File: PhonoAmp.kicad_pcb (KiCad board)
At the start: 2 copper layers, 143.5 x 76.2 mm, 33 parts, among them J1 Screw_Terminal_01x03, J2 Screw_Terminal_01x03, J3 Screw_Terminal_01x02, U1 NE5532, U2 TL072

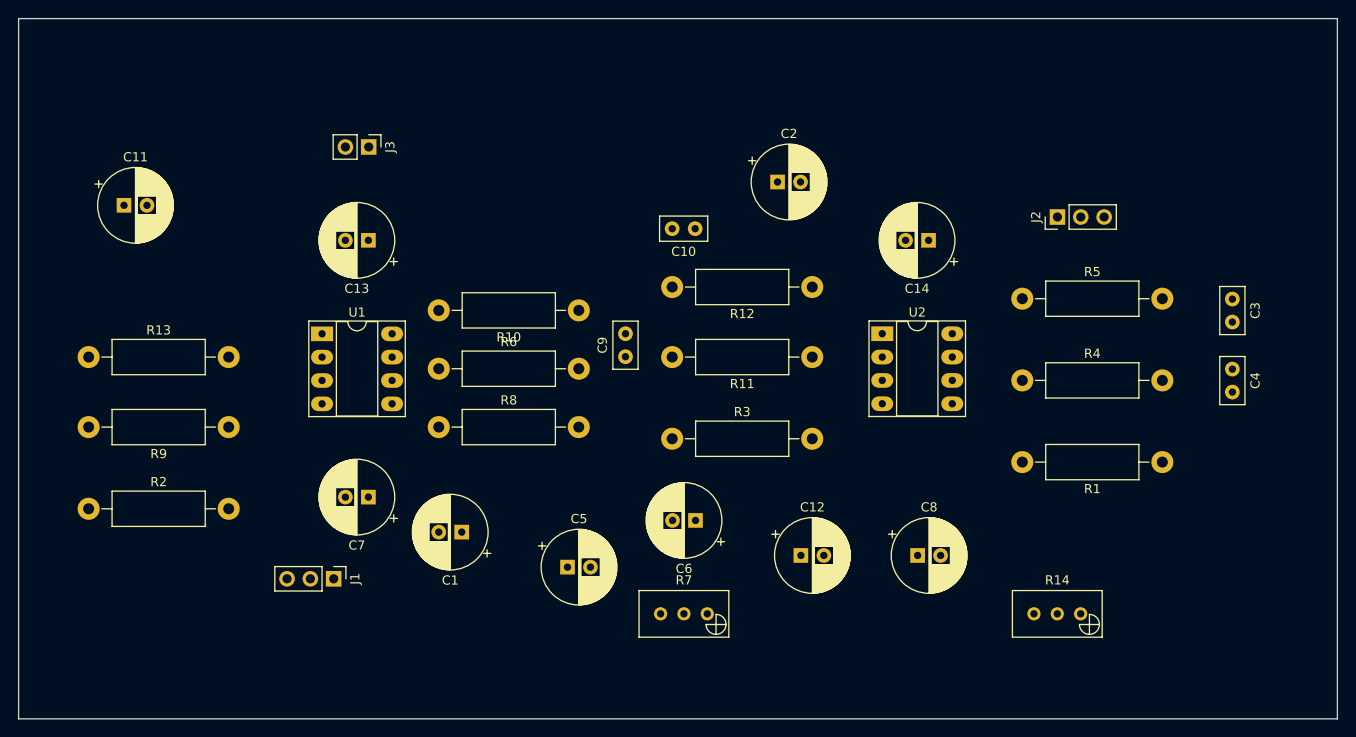
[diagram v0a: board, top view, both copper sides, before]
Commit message: Component Layout reviewed
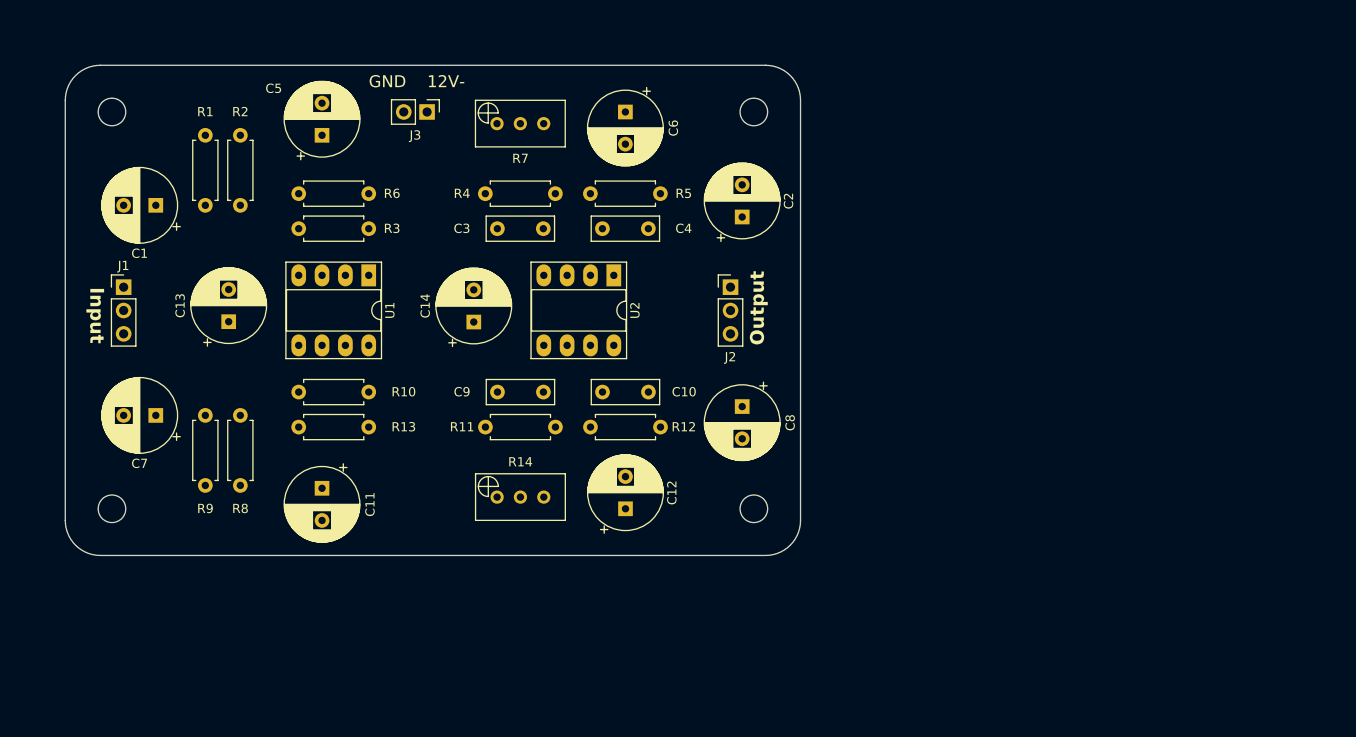
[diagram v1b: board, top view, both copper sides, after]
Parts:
- added H1: MountingHole, MountingHole:MountingHole_3mm, F.Cu at (91.4, 69.8)
- added H2: MountingHole, MountingHole:MountingHole_3mm, F.Cu at (161.3, 69.8)
- added H3: MountingHole, MountingHole:MountingHole_3mm, F.Cu at (91.4, 113.0)
- added H4: MountingHole, MountingHole:MountingHole_3mm, F.Cu at (161.3, 113.0)
- C1, C11, C12, C13, C14, C2, C5, C6, C7, C8: footprint Capacitor_THT:CP_Radial_D8.0mm_P2.50mm -> Capacitor_THT:CP_Radial_D8.0mm_P3.50mm
- C10, C3, C4, C9: footprint Capacitor_THT:C_Disc_D5.0mm_W2.5mm_P2.50mm -> Capacitor_THT:C_Rect_L7.2mm_W2.5mm_P5.00mm_FKS2_FKP2_MKS2_MKP2
- R1, R10, R11, R12, R13, R2, R3, R4, R5, R6, R8, R9: footprint Resistor_THT:R_Axial_DIN0411_L9.9mm_D3.6mm_P15.24mm_Horizontal -> Resistor_THT:R_Axial_DIN0207_L6.3mm_D2.5mm_P7.62mm_Horizontal
- moved R1 107.8 mm to (101.6, 80.0), turned to 90 degrees
- moved C3 75.4 mm to (138.4, 82.5), turned to 180 degrees
- moved C4 65.4 mm to (149.8, 82.5), turned to 180 degrees
- moved R14 64.8 mm to (133.3, 111.8), turned to 180 degrees
- moved R4 61.9 mm to (132.1, 78.7)
- moved R7 58.0 mm to (133.3, 71.1), turned to 180 degrees
- moved C5 54.1 mm to (114.3, 72.4), turned to 90 degrees
- moved C14 50.3 mm to (130.8, 92.7), turned to 90 degrees
- moved C1 48.7 mm to (96.2, 80.0)
- moved C6 45.1 mm to (147.3, 69.8), turned to -90 degrees
- moved R2 43.9 mm to (105.4, 72.4), turned to -90 degrees
- moved R5 41.0 mm to (151.1, 78.7), turned to 180 degrees
- moved R3 40.2 mm to (119.4, 82.5), turned to 180 degrees
- moved J1 39.1 mm to (92.7, 88.9), turned to 0 degrees
- moved C11 37.6 mm to (114.3, 110.8), turned to -90 degrees
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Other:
- board size 143.5 x 76.2 mm -> 80 x 53.3 mm
- board text added: "12V-"
- board text added: "GND"
- board text added: "Input"
- board text added: "Output"

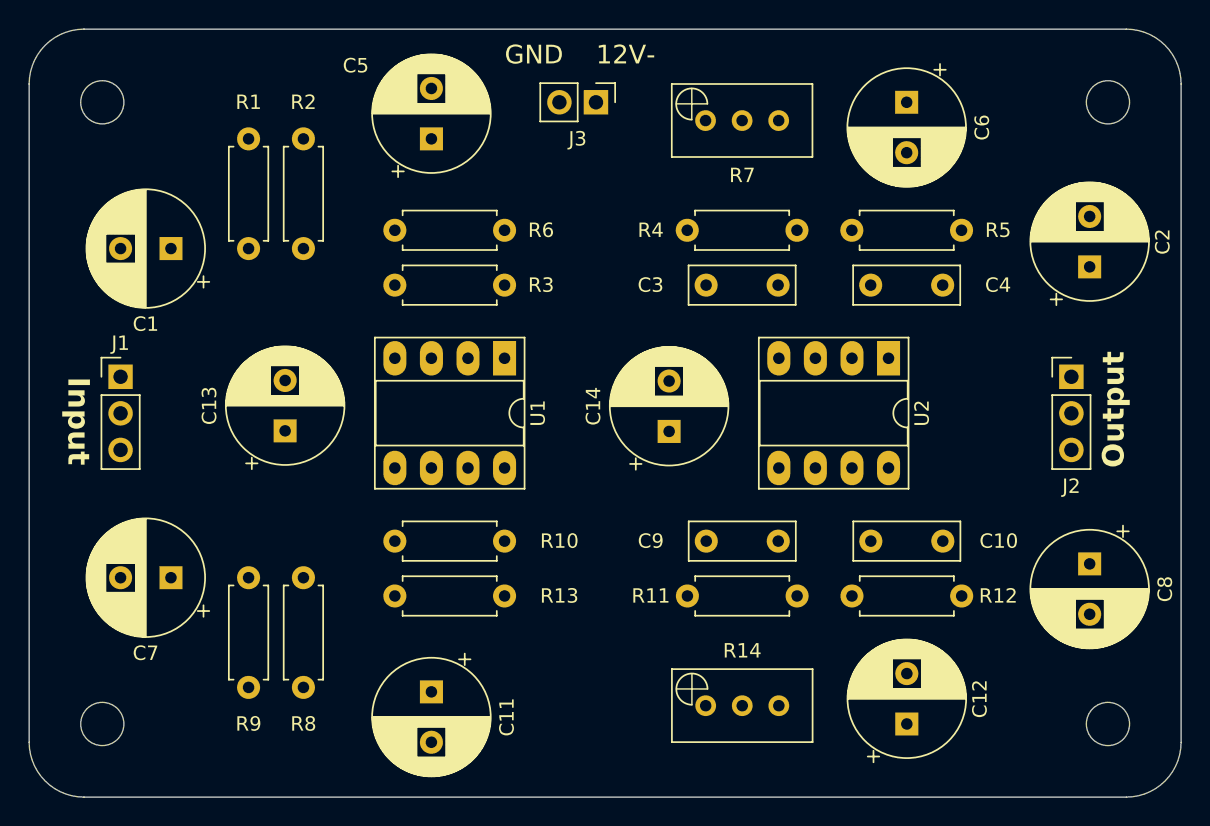
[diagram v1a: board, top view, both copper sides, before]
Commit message: iBom Production files Transferfunctions
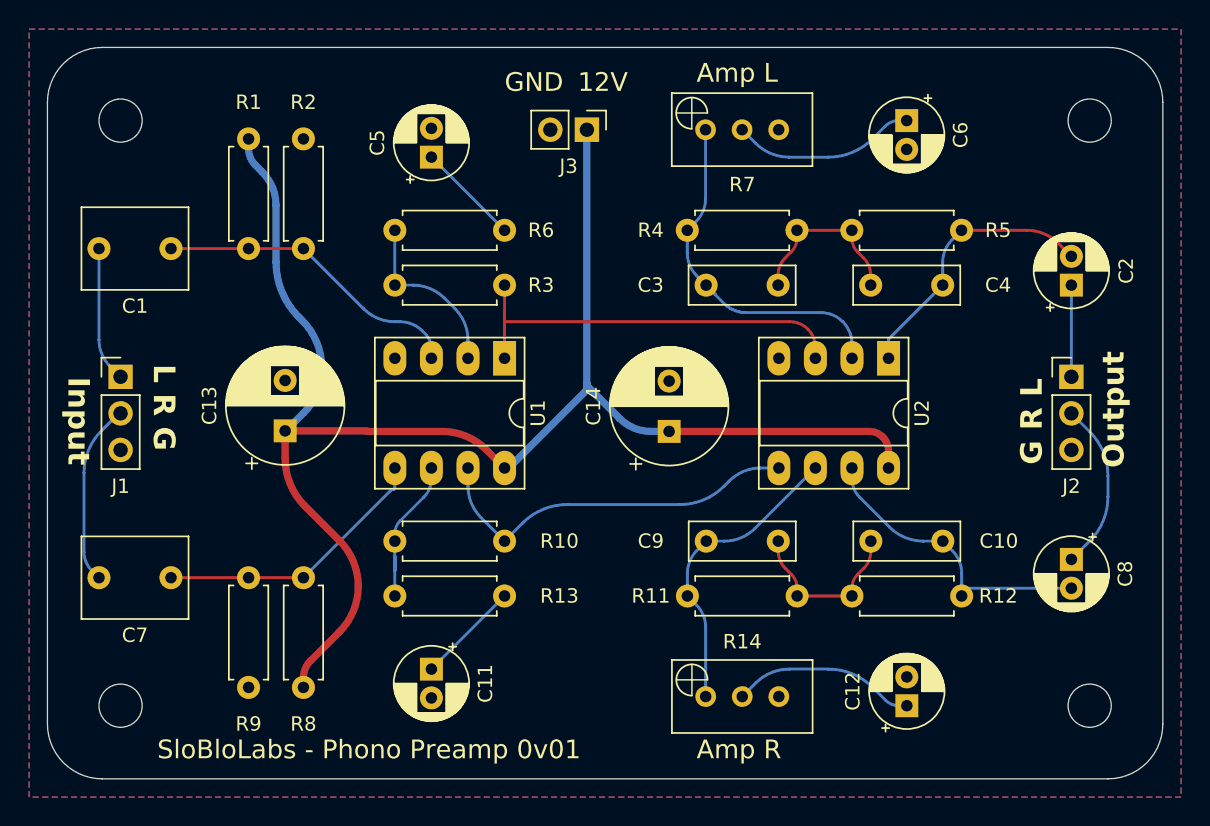
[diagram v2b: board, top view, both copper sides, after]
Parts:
- C1, C7: footprint Capacitor_THT:CP_Radial_D8.0mm_P3.50mm -> Capacitor_THT:C_Rect_L7.2mm_W5.5mm_P5.00mm_FKS2_FKP2_MKS2_MKP2
- C10, C4: value 1n5 -> 1n
- C11, C12, C2, C5, C6, C8: footprint Capacitor_THT:CP_Radial_D8.0mm_P3.50mm -> Capacitor_THT:CP_Radial_D5.0mm_P2.00mm
- C3, C9: value 6n8 -> 10n
- R11, R4: value 750k -> 1M
- moved R3 7.62 mm to (111.8, 82.5), turned to 0 degrees
- moved R6 7.62 mm to (119.4, 78.7), turned to 180 degrees
- moved J3 2.01 mm to (125.1, 71.8)
- moved C2 1.80 mm to (158.8, 82.5)
- moved H1 1.80 mm to (92.7, 71.1)
- moved H3 1.80 mm to (92.7, 111.8)
- moved H2 1.80 mm to (160.0, 71.1)
- moved H4 1.80 mm to (160.0, 111.8)
- moved C11 1.58 mm to (114.3, 109.2)
- moved C8 1.31 mm to (158.8, 101.6)
- moved C6 1.27 mm to (147.3, 71.1)
- moved C12 1.27 mm to (147.3, 111.8)
- moved C5 1.27 mm to (114.3, 73.7)
- moved R14 0.64 mm to (133.3, 111.1)
- moved R7 0.63 mm to (133.3, 71.8)
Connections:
- C1 pad 1: /op1in+ -> /op1in+L
- C10 pad 1: /op2out -> /op2outR
- C2 pad 2: /op2out -> /op2outL
- C3 pad 2: /op2in- -> /op2in-L
- C4 pad 1: /op2out -> /op2outL
- C7 pad 1: /op1in+ -> /op1in+R
- C8 pad 2: /op2out -> /op2outR
- C9 pad 2: /op2in- -> /op2in-R
- R1 pad 1: /op1in+ -> /op1in+L
- R10 pad 1: /op1in- -> /op1in-R
- R10 pad 2: /op2in+ -> /op2in+R
- R11 pad 1: /op2in- -> /op2in-R
- R12 pad 1: /op2out -> /op2outR
- R13 pad 2: /op1in- -> /op1in-R
- R14 pad 1: /op2in- -> /op2in-R
- R2 pad 2: /op1in+ -> /op1in+L
- R3 pad 1: /op1in- -> /op1in-L
- R3 pad 2: /op2in+ -> /op2in+L
- R4 pad 1: /op2in- -> /op2in-L
- R5 pad 1: /op2out -> /op2outL
- R6 pad 2: /op1in- -> /op1in-L
- R7 pad 1: /op2in- -> /op2in-L
- R8 pad 1: /op1in+ -> /op1in+R
- R9 pad 2: /op1in+ -> /op1in+R
- U1 pad 1: /op2in+ -> /op2in+L
- U1 pad 2: /op1in- -> /op1in-L
- U1 pad 3: /op1in+ -> /op1in+L
- U1 pad 5: /op1in+ -> /op1in+R
- U1 pad 6: /op1in- -> /op1in-R
- U1 pad 7: /op2in+ -> /op2in+R
- U2 pad 1: /op2out -> /op2outL
- U2 pad 2: /op2in- -> /op2in-L
- U2 pad 3: /op2in+ -> /op2in+L
- U2 pad 5: /op2in+ -> /op2in+R
- U2 pad 6: /op2in- -> /op2in-R
- U2 pad 7: /op2out -> /op2outR
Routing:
- net /12V: track 0.00 -> 109.7 mm
- net /op2in+L: track 0.00 -> 28.4 mm
- net /op2in+R: track 0.00 -> 26.6 mm
- net /op2in-L: track 0.00 -> 25.4 mm
- net /op1in+L: track 0.00 -> 21.7 mm
- net /op2outR: track 0.00 -> 21.4 mm
- net /op2in-R: track 0.00 -> 21.4 mm
- net /op1in+R: track 0.00 -> 19.5 mm
- net /op2outL: track 0.00 -> 19.1 mm
- net Net-(C12-Pad1): track 0.00 -> 12.8 mm
- net Net-(C6-Pad1): track 0.00 -> 12.8 mm
- net /input_R: track 0.00 -> 12.7 mm
- net /op1in-L: track 0.00 -> 12.2 mm
- net Net-(C3-Pad1): track 0.00 -> 11.8 mm
- net Net-(C10-Pad2): track 0.00 -> 11.8 mm
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- added copper zone on B.Cu, net GND
- added copper zone on F.Cu, net GND
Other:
- board size 80 x 53.3 mm -> 77.5 x 50.8 mm
- board text added: "12V"
- board text added: "Amp L"
- board text added: "Amp R"
- board text added: "G R L"
- board text added: "L R G"
- board text added: "SloBloLabs - Phono Preamp 0v01"
- board text removed: "12V-"
